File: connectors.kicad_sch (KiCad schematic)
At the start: 56 parts, among them J13 UART_L1, J14 UART_R1, J15 JST XH 4P, J16 JST XH 4P, J17 Conn_01x04_Male, U2 SRV05-4, U3 SRV05-4

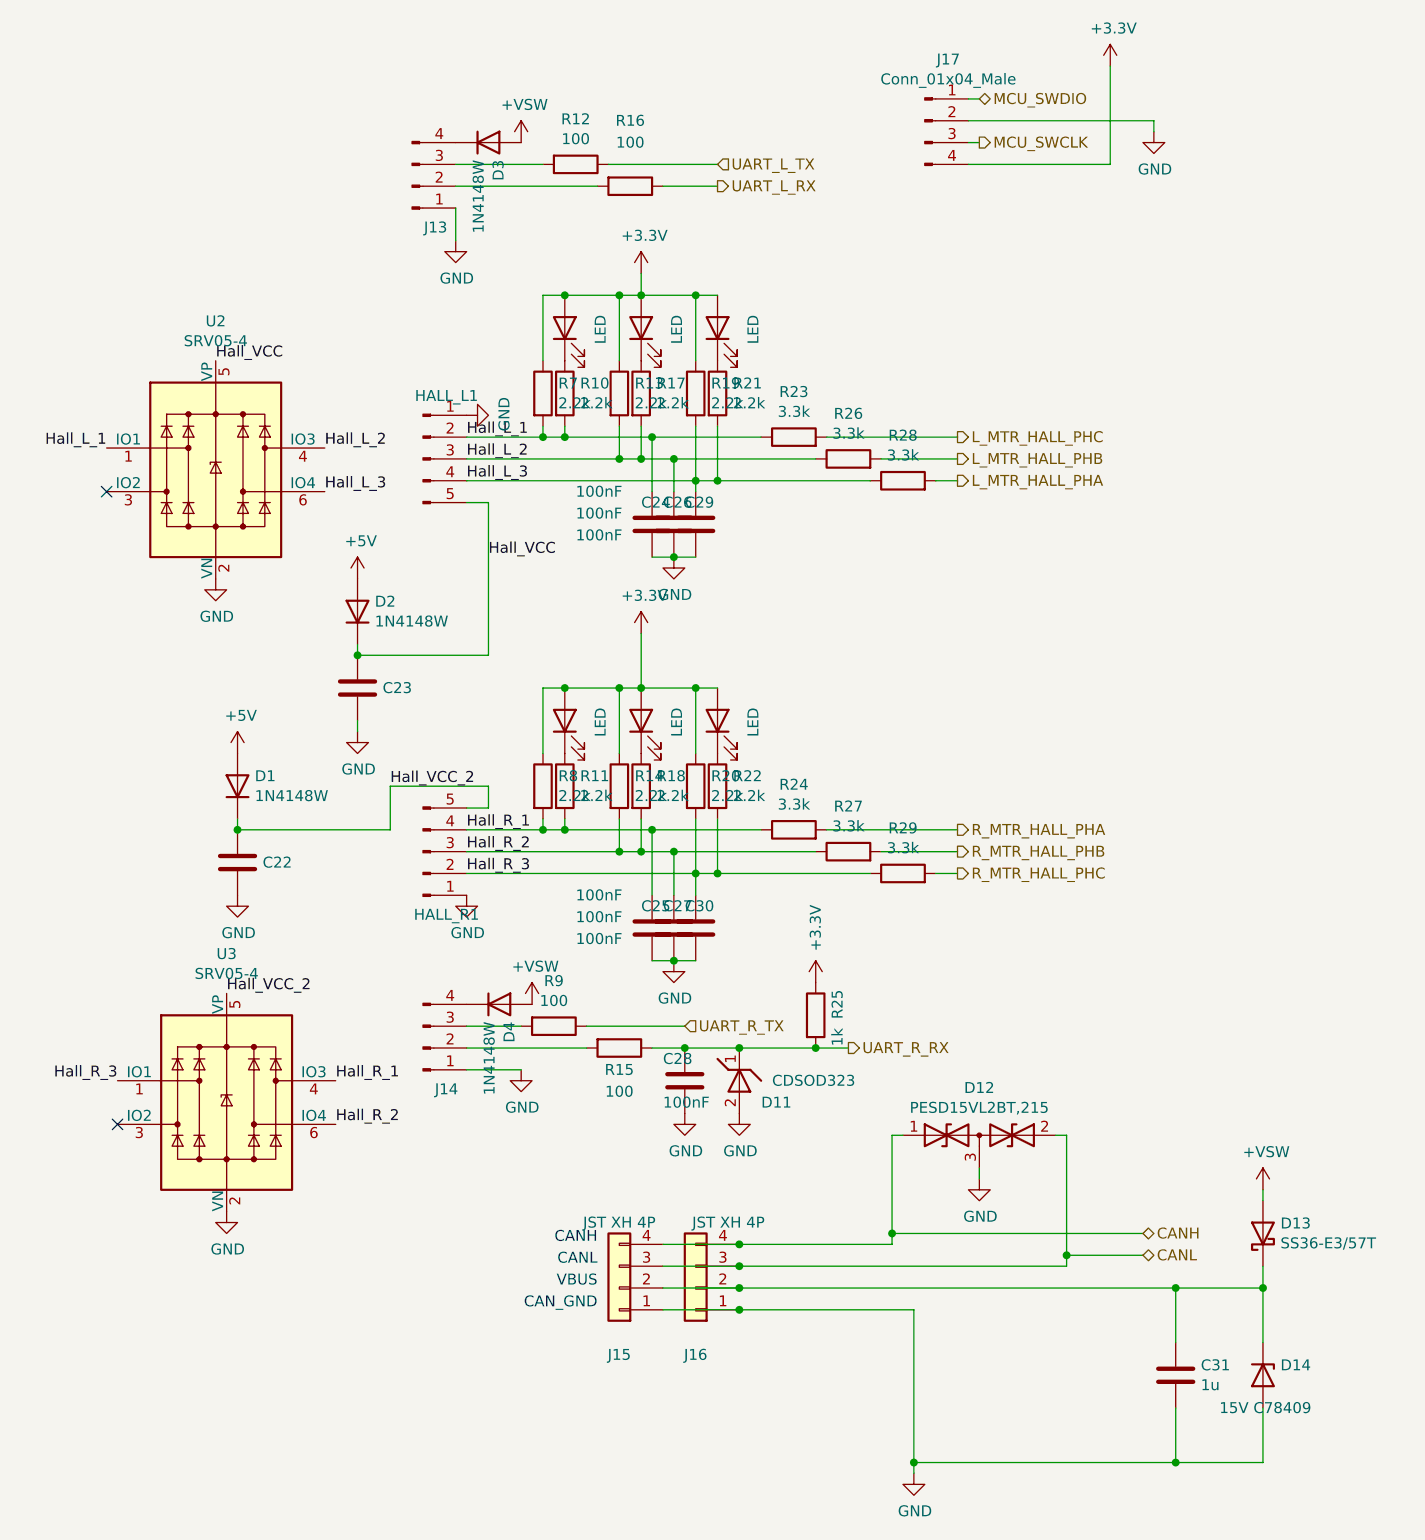
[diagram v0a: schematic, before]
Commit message: Refactor stuff adjacent to hall sensor pins
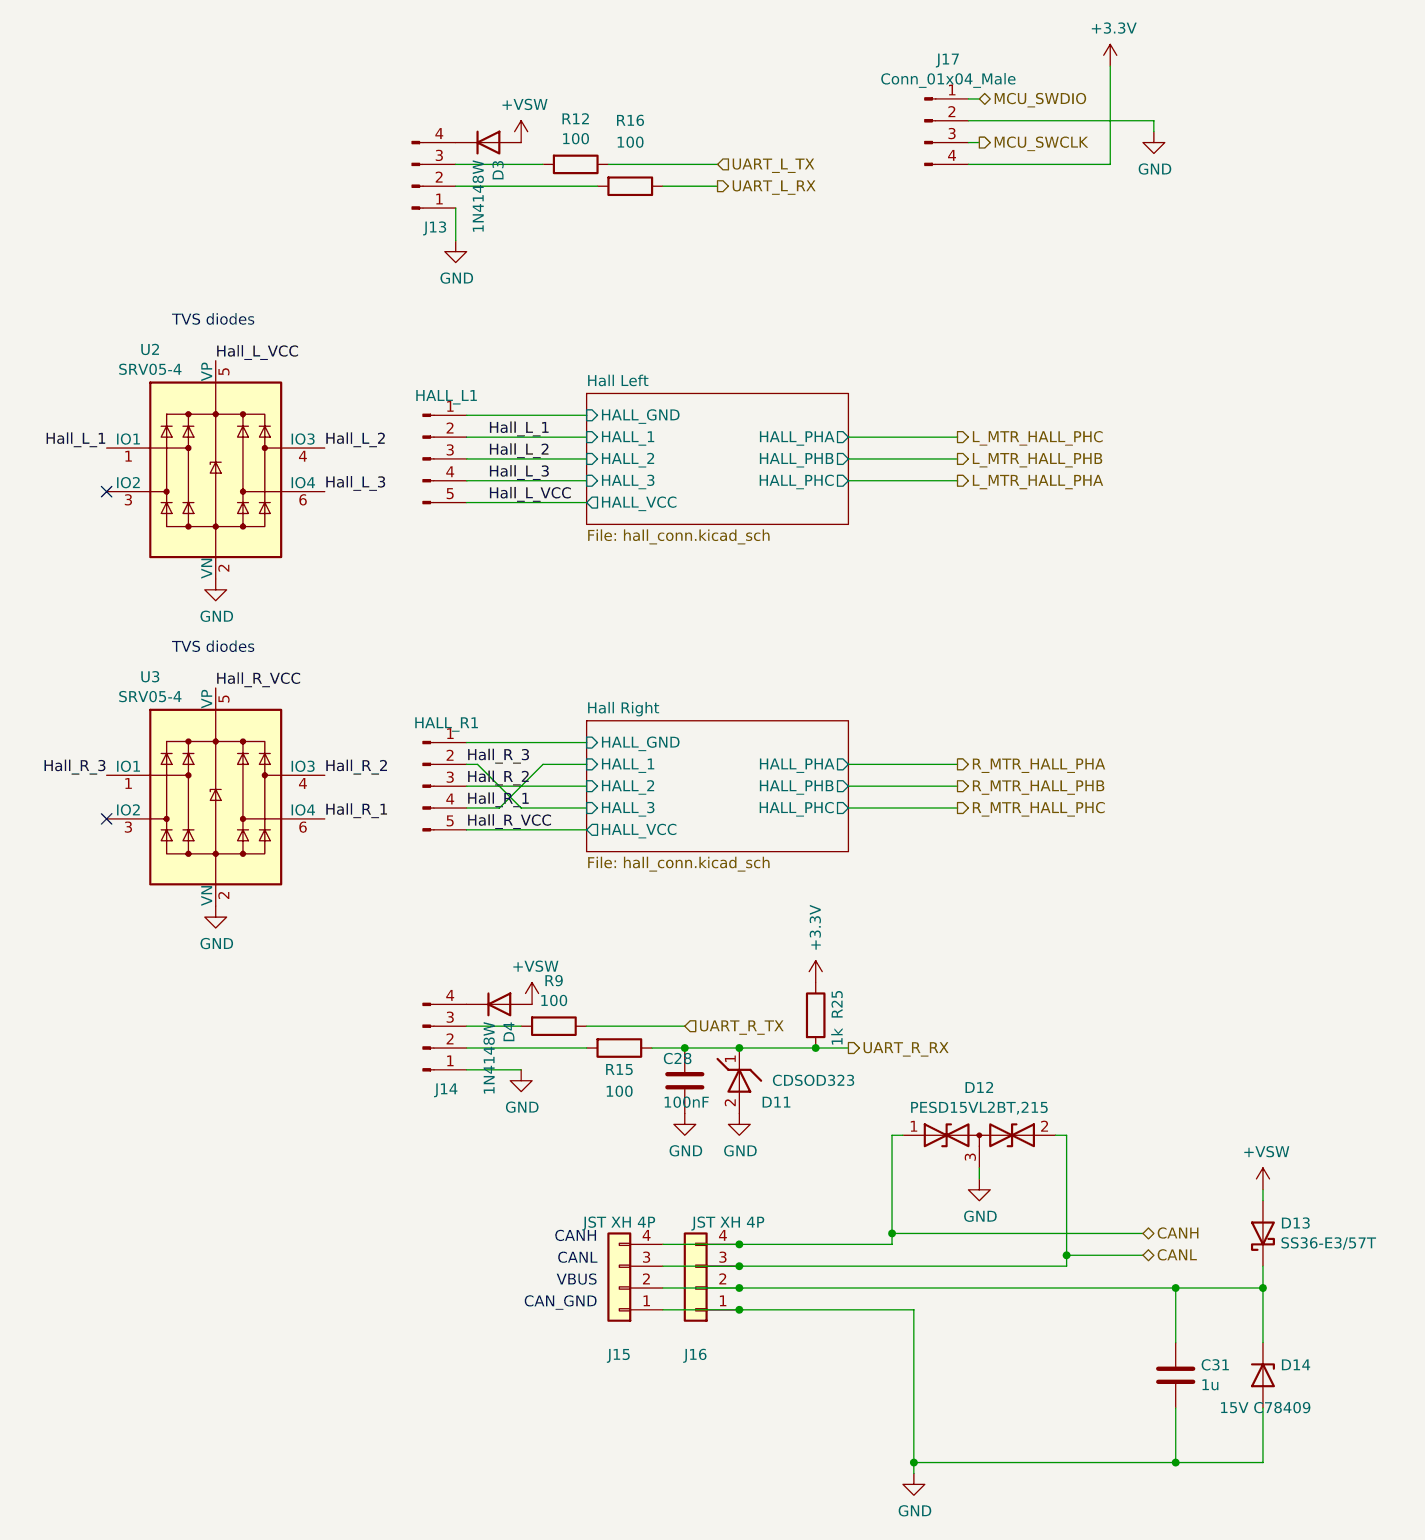
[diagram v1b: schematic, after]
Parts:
- removed C22, C23, C24, C25, C26, C27, C29, C30: 100nF, Capacitor_SMD:C_0603_1608Metric, symbol Device:C
- removed D1, D2: 1N4148W, Diode_SMD:D_SOD-123, symbol Device:D
- removed D10, D5, D6, D7, D8, D9: LED, LED_SMD:LED_0603_1608Metric, symbol Device:LED
- removed R10, R11, R13, R14, R17, R18, R19, R20, R21, R22, R7, R8: 2.2k, Resistor_SMD:R_0603_1608Metric, symbol Device:R
- removed R23, R24, R26, R27, R28, R29: 3.3k, Resistor_SMD:R_0603_1608Metric, symbol Device:R
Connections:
- net GND: no longer HALL_L1.1 (Pin_1), HALL_R1.1 (Pin_1)
- net Hall_R_1: now also U3.6 (IO4); no longer U3.4 (IO3)
- net Hall_R_2: now also U3.4 (IO3); no longer U3.6 (IO4)
- net Hall_VCC renamed Hall_L_VCC
- net Hall_VCC_2 renamed Hall_R_VCC
- new net Hall Left/HALL_GND: HALL_L1.1 (Pin_1)
- new net Hall Right/HALL_GND: HALL_R1.1 (Pin_1)
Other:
- added sheet Hall Left (hall_conn.kicad_sch)
- added sheet Hall Right (hall_conn.kicad_sch)
- note added: "TVS diodes"
- moved on the sheet: HALL_R1

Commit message: Update a few library symbols
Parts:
- D12: symbol Device:D_TVS_x2_AAC -> Device:D_TVS_Dual_AAC
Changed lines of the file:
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@@
     (pin "2")
   )
-  (symbol (lib_id "Device:D_TVS_x2_AAC") (at 125.73 149.86 0) (unit 1)
+  (symbol (lib_id "Device:D_TVS_Dual_AAC") (at 125.73 149.86 0) (unit 1)
     (in_bom yes) (on_board yes)
     (property "Reference" "D12" (id 0) (at 125.73 144.3482 0))
